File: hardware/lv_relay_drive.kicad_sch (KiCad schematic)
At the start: 21 parts, among them Q3 NMOS, Q5 NMOS, Q6 NMOS

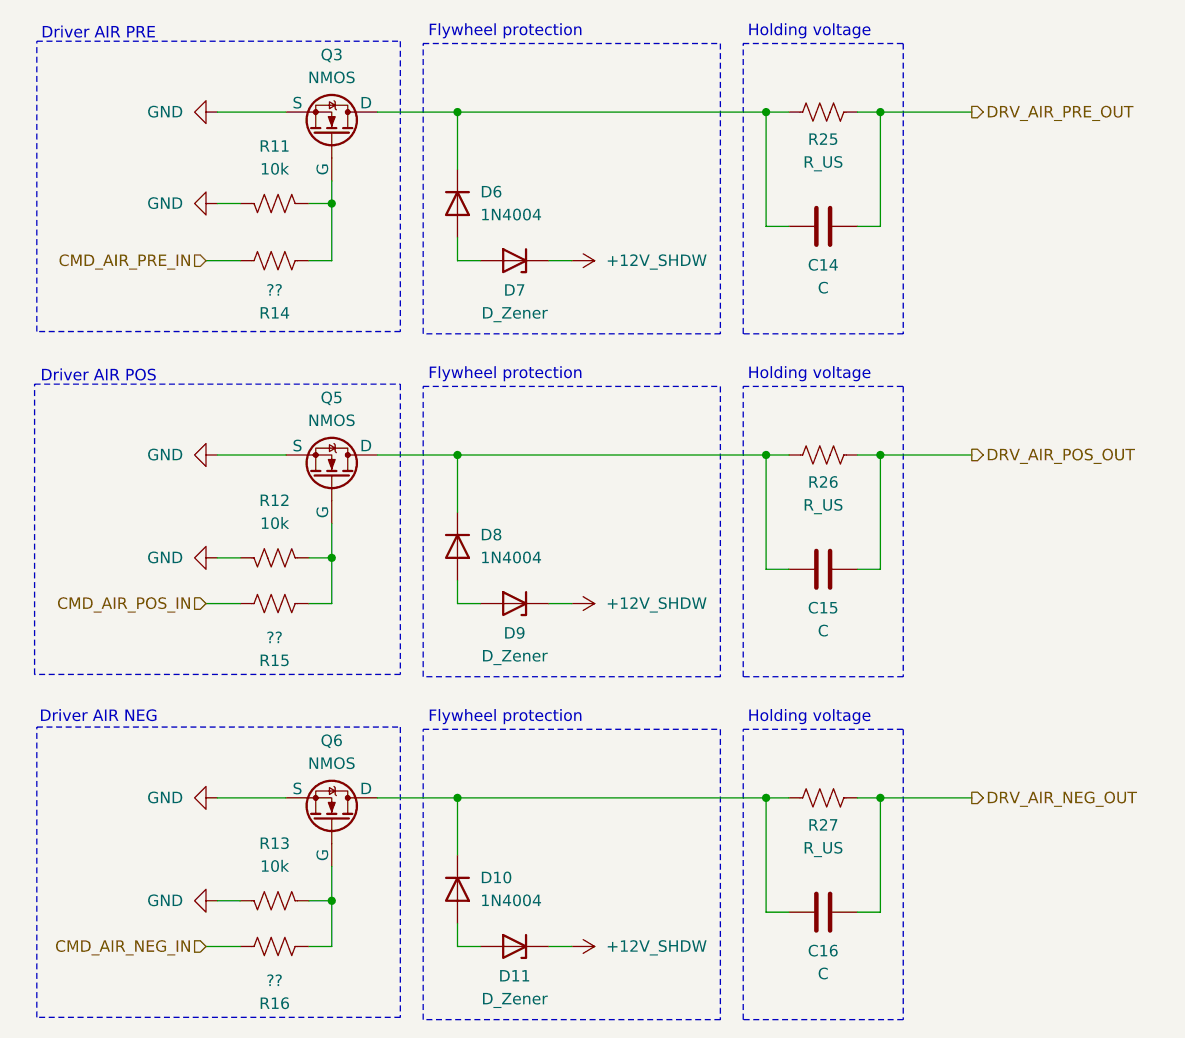
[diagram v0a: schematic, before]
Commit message: start power supply and logic sizing
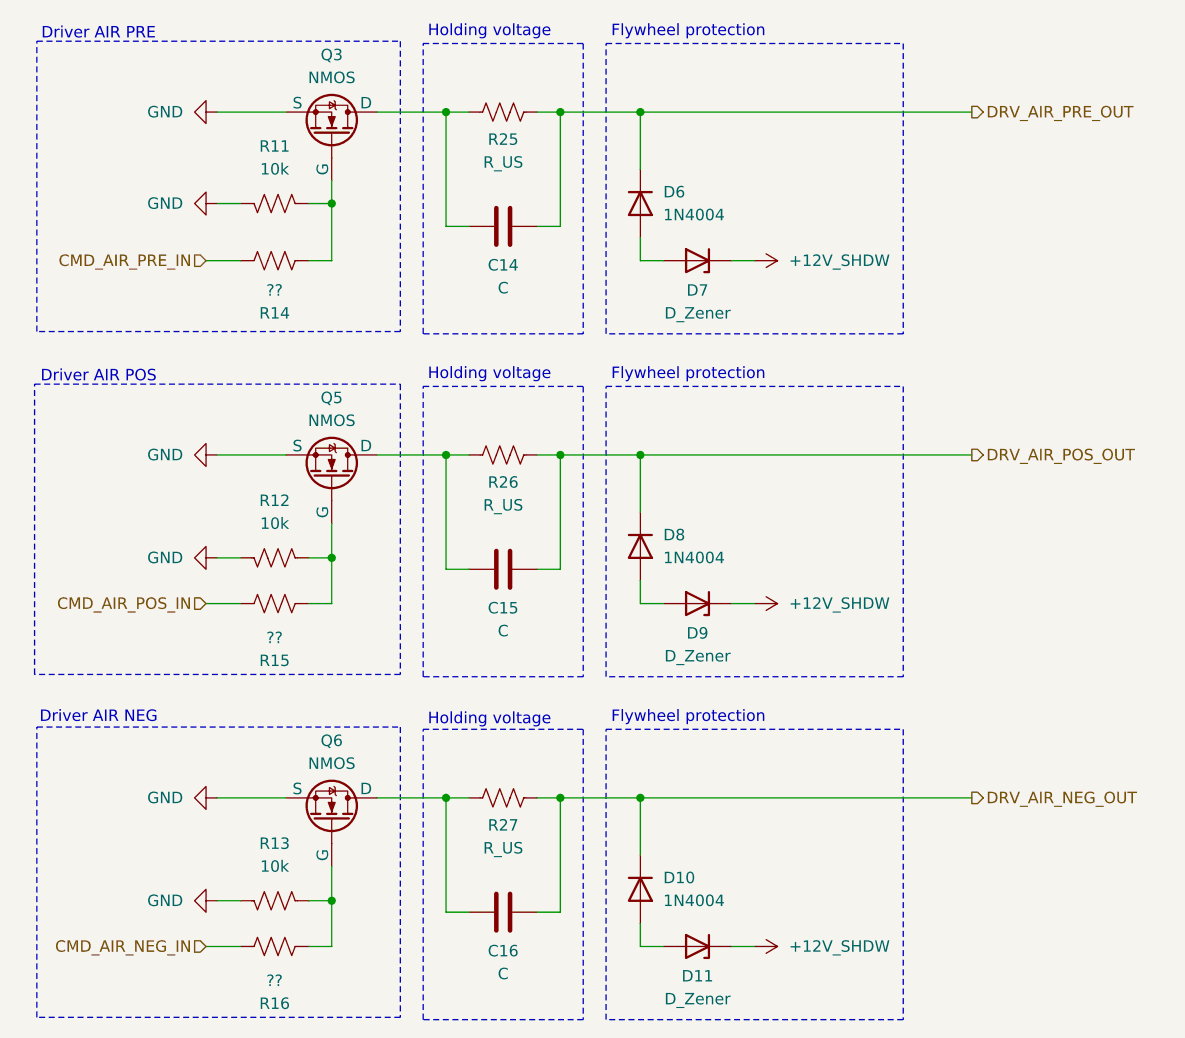
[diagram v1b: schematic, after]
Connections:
- net DRV_AIR_NEG_OUT: now also D10.1 (K)
- net DRV_AIR_POS_OUT: now also D8.1 (K)
- net DRV_AIR_PRE_OUT: now also D6.1 (K)
- net at C14.2, Q3.1 (D), R25.1: no longer D6.1 (K)
- net at C15.2, Q5.1 (D), R26.1: no longer D8.1 (K)
- net at C16.2, Q6.1 (D), R27.1: no longer D10.1 (K)
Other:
- moved on the sheet: C14, C15, C16, R25, R26, R27
